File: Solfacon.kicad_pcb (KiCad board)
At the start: 2 copper layers, 48 x 73 mm, 50 parts, among them Q1 TSM480P06, Q2 TP0606, Q3 ZVN3306A, Q4 STP55NF06L, U1 ATtiny85

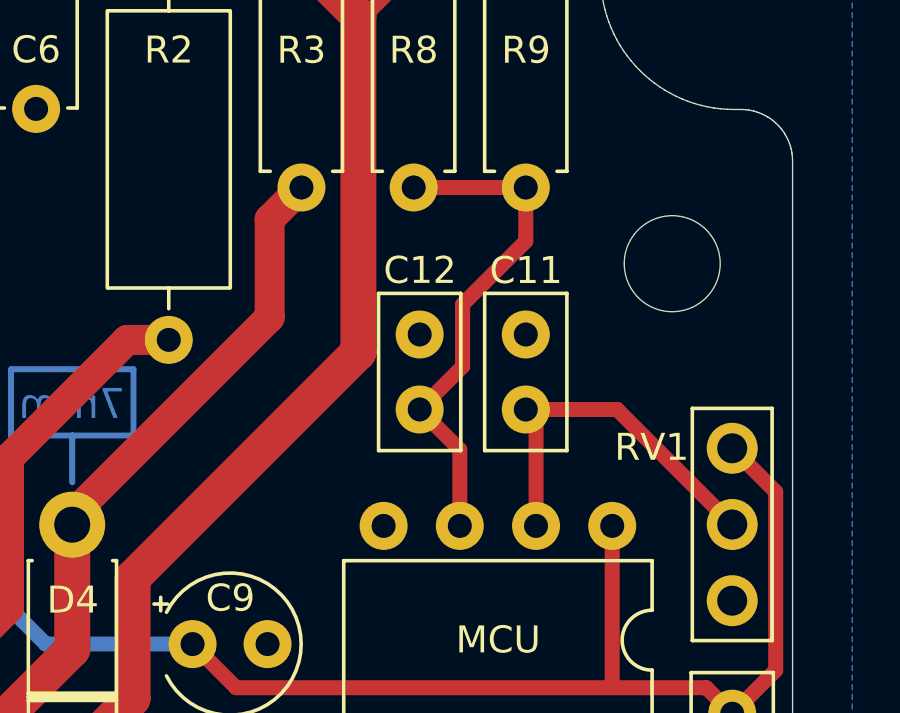
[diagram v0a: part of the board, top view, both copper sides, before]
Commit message: Add files via upload
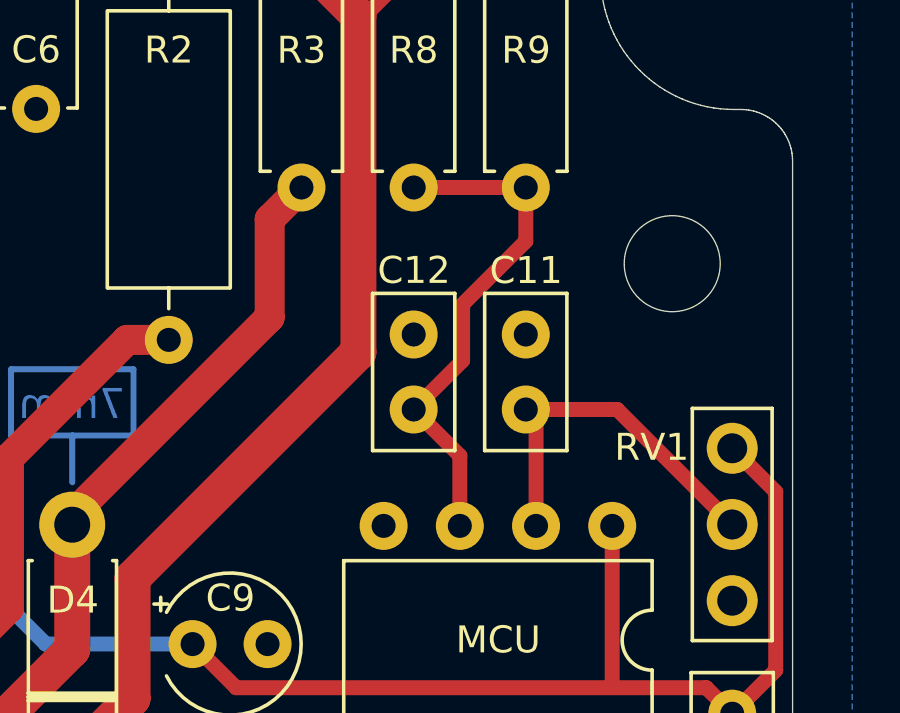
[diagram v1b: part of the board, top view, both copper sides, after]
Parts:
- D5: value 1N5817 -> SB140
- R1, R5: value 47K -> 22K
- R3: value 330 -> 200
- moved C12 0.20 mm to (65.4, 46.5)
